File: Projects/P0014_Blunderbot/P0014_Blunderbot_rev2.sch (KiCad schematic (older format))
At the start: 20 parts, among them J1 22-03-5035, J2 22-03-5035, J3 70553-0037, J4 70553-0037, J5 CONN_01X04, J6 CONN_01X04, P1 CONN_02X03, U1 TC7W241FUTE12LF, U2 MIC5219-5.0YM5-TR, U3 MIC5219-5.0YM5-TR, U4 ATTINY841-SSU

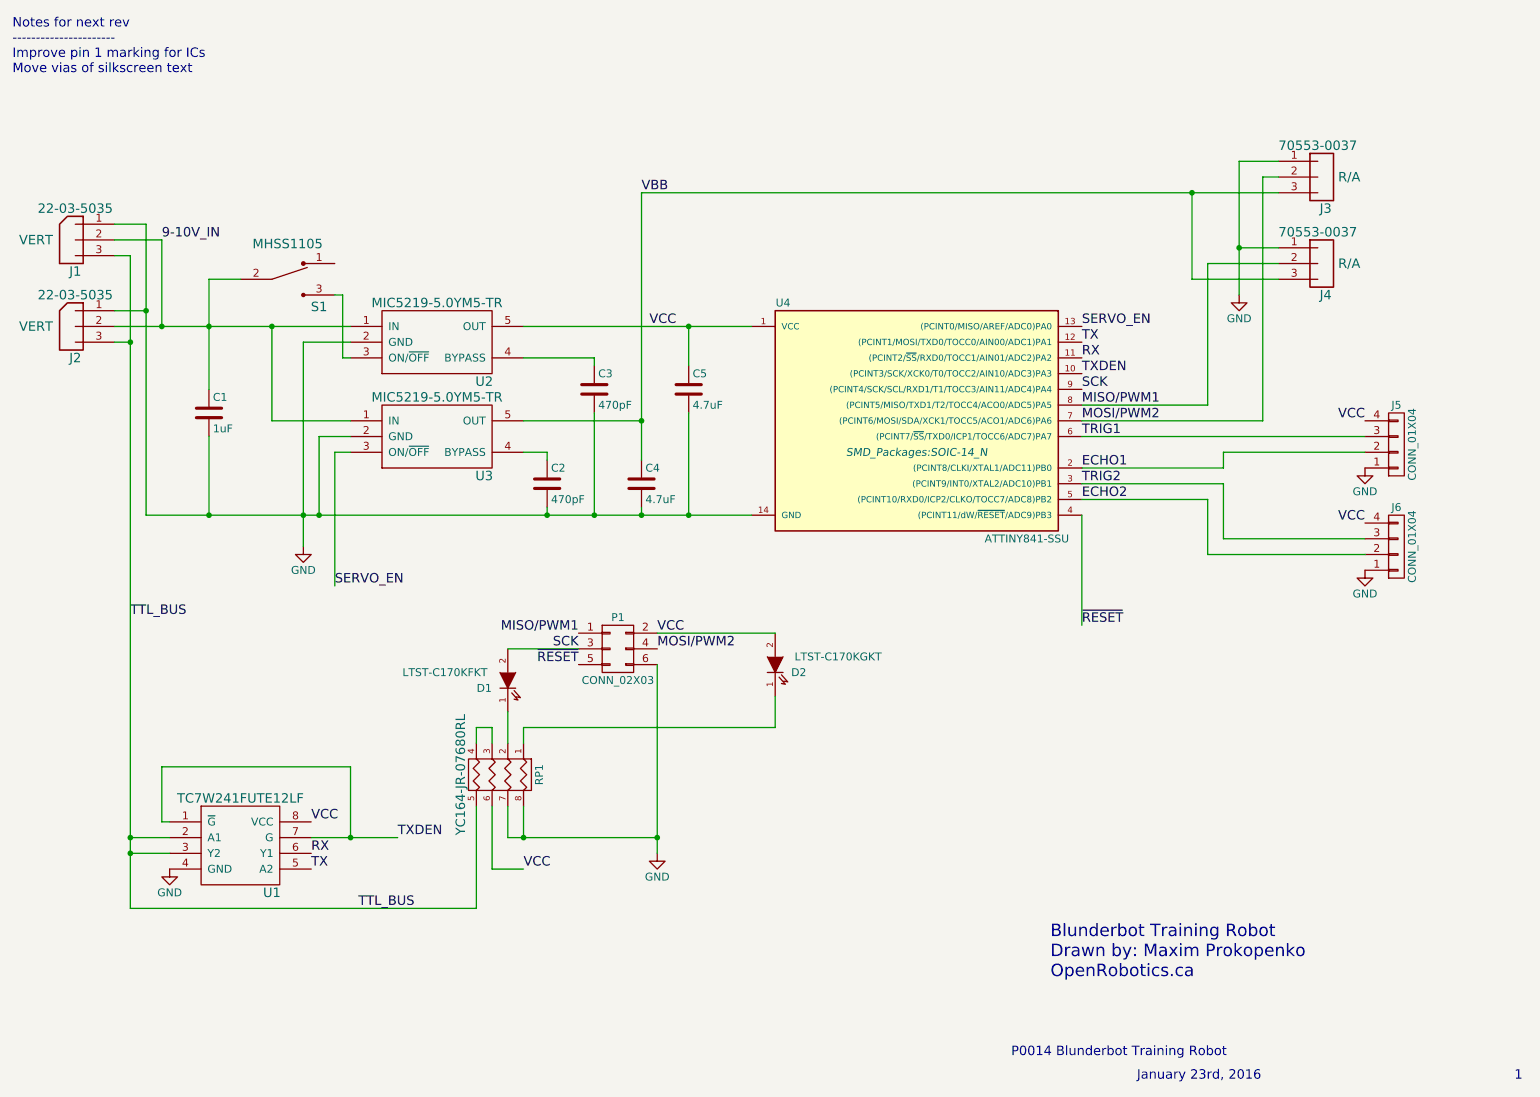
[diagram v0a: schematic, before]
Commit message: Started rev2
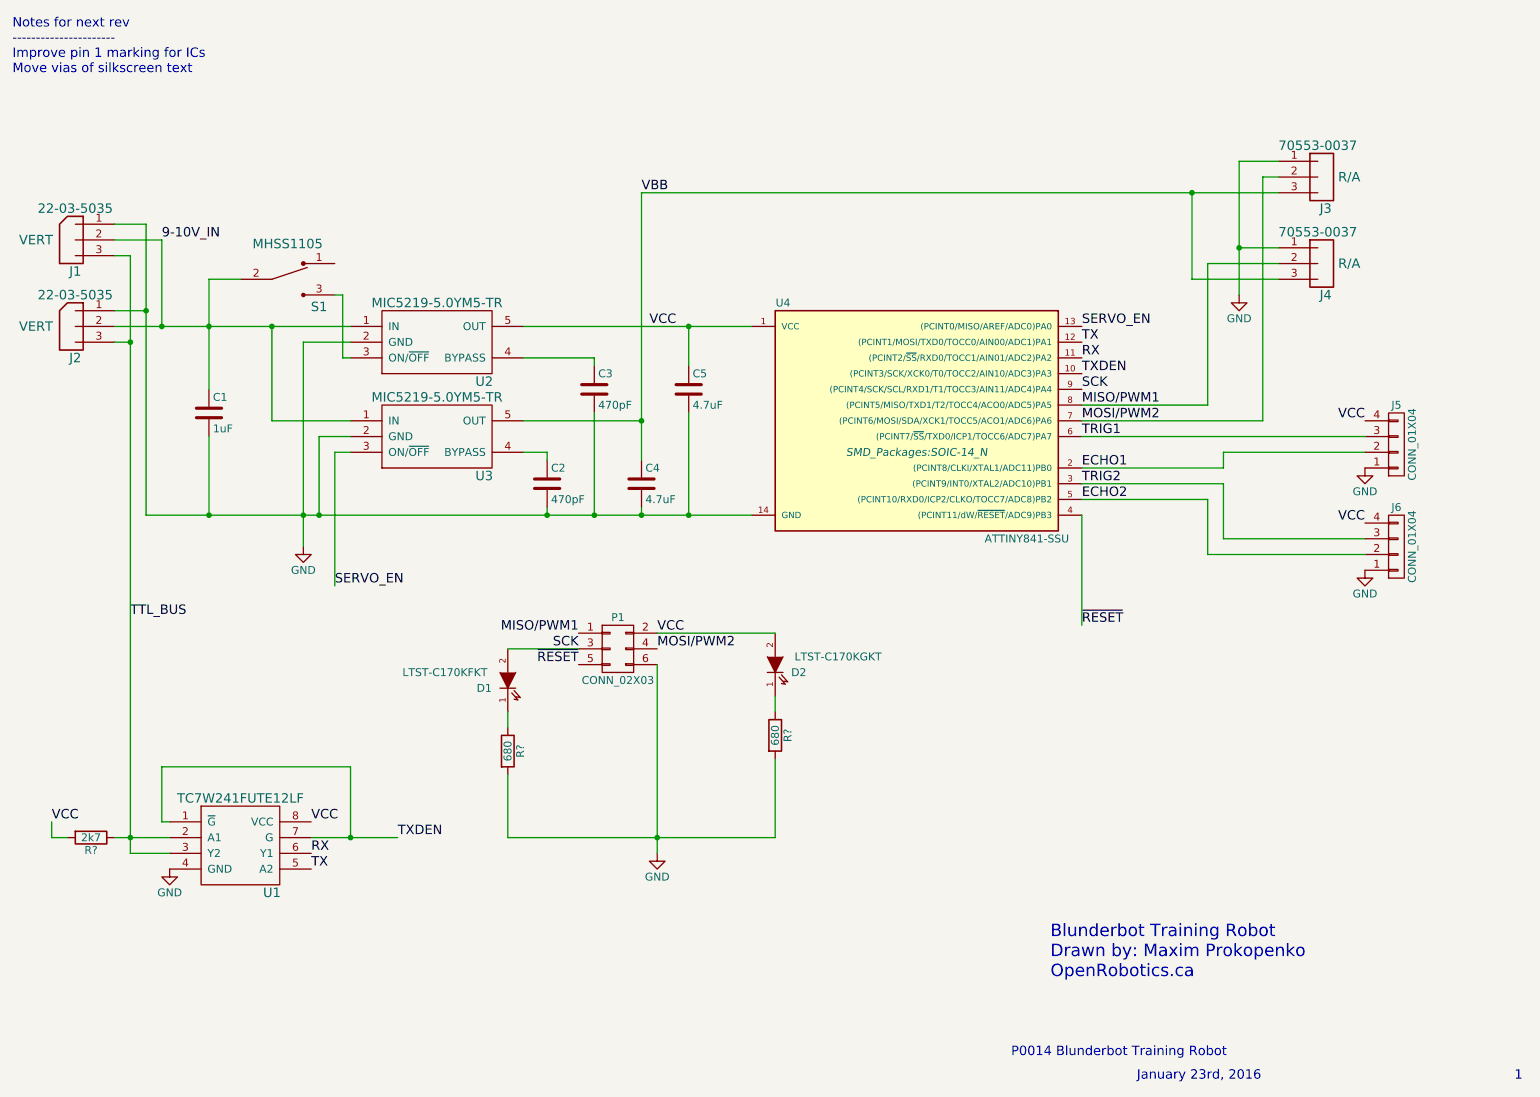
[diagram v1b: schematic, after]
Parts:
- removed RP1: YC164-JR-07680RL, Resistors_SMD:R_Array_Convex_4x1206, symbol R_PACK4
- added R?: 2k7, symbol R
- added R? (x2): 680, symbol R
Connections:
- net GND: now also R?.2, R?.2
- net TTL_BUS: now also R?.1
- net VCC: now also R?.2
- net at D2.1 (K): now also R?.1
- net at D1.1 (K): now also R?.1
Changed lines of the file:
@@
 Data
 89 50 4E 47 0D 0A 1A 0A 00 00 00 0D 49 48 44 52 00 00 00 84 00 00 00 84 08 03 00 00 00 66 9A 73
-95 00 00 00 03 73 42 49 54 08 08 08 DB E1 4F E0 00 00 01 71 50 4C 54 45 02 00 00 5B 5B 5C 2B 2B
+95 00 00 00 03 73 42 49 54 08 08 08 DB E1 4F E0 00 00 01 71 50 4C 54 45 01 00 00 5B 5B 5C 2B 2B
 2B 22 07 09 34 0A 0E 3A 0B 0F 29 25 25 2B 09 0C 24 0B 0D 34 34 34 68 67 68 3A 3A 3B 4C 0D 13 6B
 12 1B 9C 1A 26 B4 1D 2C BF 1E 2E 7F 16 20 63 64 64 AB 1C 2A 8E 18 23 64 11 19 3E 0B 10 1E 13 14
@@
 1C 3E 3F 40 4E 51 53 6F 6F 70 80 7F 80 0F 10 10 2E 2F 30 0F 0F 10 57 5A 5C E0 DF E0 46 4A 4C 17
 18 18 5C 5E 60 B7 B8 B9 BE BE C0 1F 1F 20 8F 8F 90 1D 0B 0C 27 28 29 1E 0F 10 46 47 48 26 1F 20
-2F 30 31 37 38 39 75 73 74 78 36 5E 62 00 00 00 01 74 52 4E 53 00 40 E6 D8 66 00 00 15 0B 49 44
+2F 30 31 37 38 39 75 73 74 DC 64 69 7C 00 00 00 01 74 52 4E 53 00 40 E6 D8 66 00 00 15 0B 49 44
 41 54 78 9C BD 5C 89 43 DA CA D6 57 5C 30 B2 16 C4 85 BA 57 45 6D 4B AD 20 54 33 2C B5 22 8B 95
 0C 52 54 52 4B 31 54 11 2B B6 F4 F5 76 F9 FE FA EF CC 4C 42 16 02 F6 F2 EE 7D A7 6A 60 92 CC F9
@@
 AA 3A 6B 5E F4 95 4C FE 1D FA A9 32 D3 19 7D E8 45 BB BD 3F FF FC B7 88 B3 FA 26 A8 E8 67 96 74
 ED F2 03 04 D7 8C BD EF F7 21 FF 16 CD 72 7F D9 E7 1D 06 27 B8 66 9F 98 F0 8D 4C 71 83 E6 F7 FC
-AF 68 BC EF FF 0B E4 FF 01 8C 6E BB 14 85 49 1E 74 00 00 00 00 49 45 4E 44 AE 42 60 82 A0
+AF 68 BC EF FF 0B E4 FF 01 8C 6E BB 14 85 49 1E 74 00 00 00 00 49 45 4E 44 AE 42 60 82 8C
 EndData
 $EndBitmap
@@
 Wire Wire Line
 	1650 2400 1750 2400
-Wire Wire Line
-	1750 2400 1750 6550
 Wire Wire Line
 	1750 2950 1650 2950
@@
 MOSI/PWM2
 Wire Wire Line
-	5850 5200 5850 5400
-Wire Wire Line
-	4150 5300 4150 5500
-Wire Wire Line
-	4150 5900 4150 6100
-Wire Wire Line
 	5100 5000 5100 6200
 $Comp
@@
 Text Label 3450 6100 0    60   ~ 0
 TXDEN
-Wire Wire Line
-	3950 5900 3950 6550
-Wire Wire Line
-	3950 6550 1750 6550
-Connection ~ 1750 6200
 $Comp
 L GND #PWR06
@@
 	1    0    0    -1
 $EndComp
-Text Label 4250 6300 0    60   ~ 0
+Text Label 1250 6000 0    60   ~ 0
 VCC
 Text Label 9600 3450 2    60   ~ 0
@@
 Text Label 1750 4700 0    60   ~ 0
 TTL_BUS
-$Comp
-L R_PACK4 RP1
-U 1 1 56AF2196
-P 3900 5700
-F 0 "RP1" H 3900 6150 50  0000 C CNN
-F 1 "YC164-JR-07680RL" H 3900 5650 60  0000 C CNN
-F 2 "Resistors_SMD:R_Array_Convex_4x1206" H 3900 5700 50  0001 C CNN
-F 3 "" H 3900 5700 50  0000 C CNN
-F 4 "YC164-JR-07680RL" H 3900 5650 60  0001 C CNN "Part1"
-	1    3900 5700
-	0    1    1    0
-$EndComp
-Wire Wire Line
-	2000 6200 1750 6200
-Wire Wire Line
-	4250 5500 4250 5400
-Wire Wire Line
-	4250 5400 5850 5400
-Wire Wire Line
-	4250 5900 4250 6100
-Wire Wire Line
-	4150 6100 5100 6100
+Wire Wire Line
+	1750 6200 2000 6200
 Connection ~ 5100 6100
-Connection ~ 4250 6100
-Wire Wire Line
-	3950 5400 4050 5400
-Wire Wire Line
-	4050 5400 4050 5500
-Wire Wire Line
-	4050 5900 4050 6300
-Wire Wire Line
-	4050 6300 4250 6300
-Text Label 3200 6550 0    60   ~ 0
-TTL_BUS
-Wire Wire Line
-	3950 5500 3950 5400
 Wire Wire Line
 	9050 1900 8950 1900
@@
 	8950 3450 7800 3450
 Wire Wire Line
-	2000 6100 1750 6100
+	1650 6100 2000 6100
 Connection ~ 1750 6100
 Text Notes 1000 1250 0    60   ~ 0
 Notes for next rev\n----------------------\nImprove pin 1 marking for ICs\nMove vias of silkscreen text
+$Comp
+L R R?
+U 1 1 57B67C25
+P 1500 6100
+F 0 "R?" V 1580 6100 50  0000 C CNN
+F 1 "2k7" V 1500 6100 50  0000 C CNN
+F 2 "" V 1430 6100 50  0000 C CNN
+F 3 "" H 1500 6100 50  0000 C CNN
+	1    1500 6100
+	0    1    1    0
+$EndComp
+Wire Wire Line
+	1350 6100 1250 6100
+Wire Wire Line
+	1250 6100 1250 6000
+Wire Wire Line
+	1750 2400 1750 6200
+$Comp
+L R R?
+U 1 1 57B68C7E
+P 5850 5450
+F 0 "R?" V 5930 5450 50  0000 C CNN
+F 1 "680" V 5850 5450 50  0000 C CNN
+F 2 "" V 5780 5450 50  0000 C CNN
+F 3 "" H 5850 5450 50  0000 C CNN
+	1    5850 5450
+	1    0    0    -1
+$EndComp
+$Comp
+L R R?
+U 1 1 57B68D4E
+P 4150 5550
+F 0 "R?" V 4230 5550 50  0000 C CNN
+F 1 "680" V 4150 5550 50  0000 C CNN
+F 2 "" V 4080 5550 50  0000 C CNN
+F 3 "" H 4150 5550 50  0000 C CNN
+	1    4150 5550
+	1    0    0    -1
+$EndComp
+Wire Wire Line
+	4150 5400 4150 5300
+Wire Wire Line
+	4150 5700 4150 6100
+Wire Wire Line
+	4150 6100 5850 6100
+Wire Wire Line
+	5850 6100 5850 5600
+Wire Wire Line
+	5850 5300 5850 5200
 $EndSCHEMATC
